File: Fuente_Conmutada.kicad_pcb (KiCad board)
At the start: 2 copper layers, 135 x 85 mm, 54 parts, among them J1 Terminal_220v, J2 Terminal_12v, J3 Vout, Q1 IRF840, Q2 IRF840, T1 Transformer_1P_SS, U1 TL494, U2 IR2110

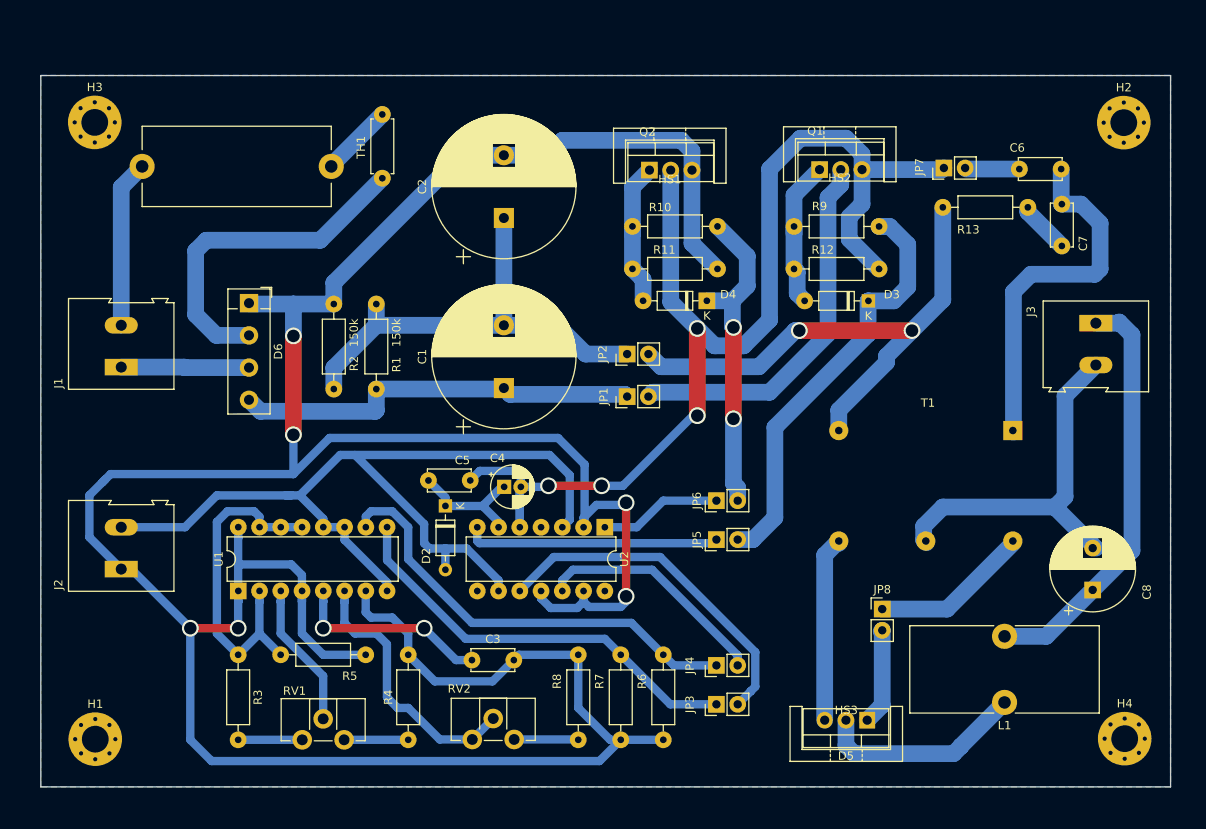
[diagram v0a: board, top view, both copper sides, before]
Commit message: huj
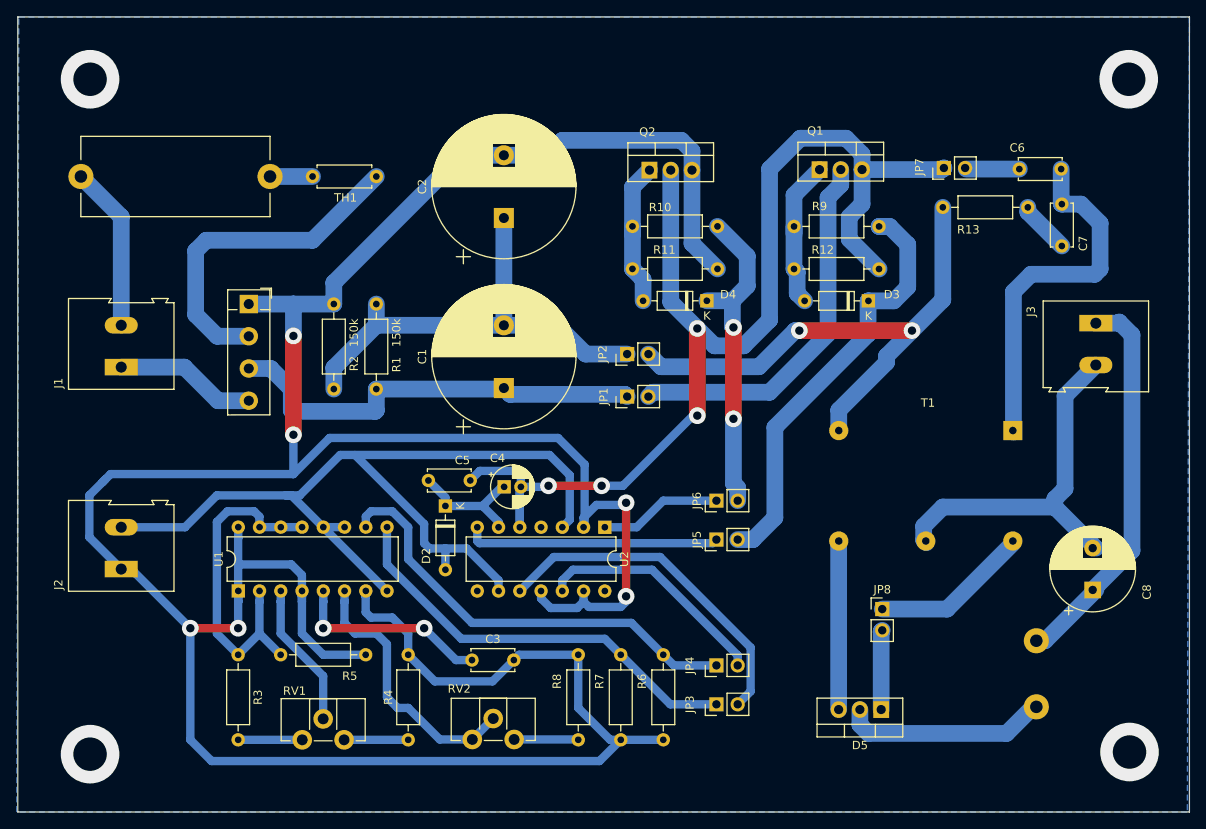
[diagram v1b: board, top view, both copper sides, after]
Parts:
- removed D6: B40C2300-1500A, Diode_THT:Diode_Bridge_Vishay_KBPM
- removed H1, H2, H3, H4: MountingHole_Pad, MountingHole:MountingHole_3.2mm_M3_Pad_Via
- removed HS1, HS2, HS3: Heatsink, Heatsink:Heatsink_Stonecold_HS-S01_13.21x6.35mm
- added D1: B80C2300-1500B, Diode_THT:Diode_Bridge_Vishay_KBPM, F.Cu at (101.0, 75.2)
- L1: moved to B.Cu
- moved F1 7.41 mm to (103.5, 60.0)
- moved L1 3.84 mm to (195.1, 123.3), turned to 0 degrees
- moved D5 2.10 mm to (176.6, 123.7)
- moved TH1 0.74 mm to (116.2, 60.0), turned to 180 degrees
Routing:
- net Net-(F1-Pad1): track 8.74 -> 5.08 mm
- net Net-(J3-Pin_1): track 50.3 -> 47.1 mm
- net Net-(D1-+): track 48.8 -> 51.9 mm
- net Net-(D5-A2): track 22.2 -> 20.0 mm
- net Net-(D5-A1): track 11.7 -> 9.52 mm
- net GND_AC: track 15.3 -> 16.9 mm
- net +12V: track 111.1 -> 112.6 mm
- net Net-(D1-Pad2): track 40.9 -> 40.3 mm
- net (no net): vias 0 -> 4
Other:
- board size 135 x 85 mm -> 140 x 95 mm
